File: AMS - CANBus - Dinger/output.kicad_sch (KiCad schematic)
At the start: 7 parts, among them Q3 2N7000, Q4 IRF9Z34NPBF

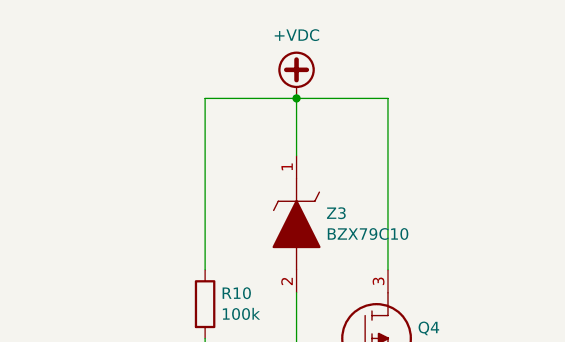
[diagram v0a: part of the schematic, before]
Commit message: initial placement of parts
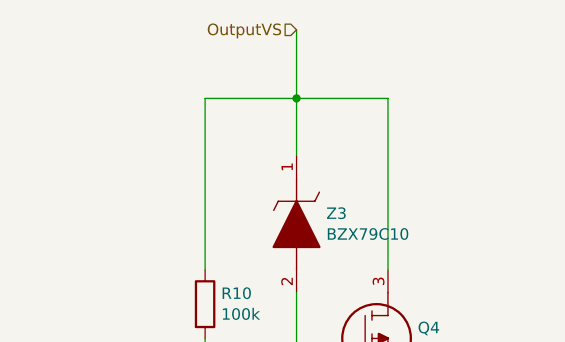
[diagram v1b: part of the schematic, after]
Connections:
- net +VDC renamed OutputVS
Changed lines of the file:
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@@
+	(wire
+		(pts
+			(xy 130.81 54.61) (xy 130.81 62.23)
+		)
+		(stroke
+			(width 0)
+			(type default)
+		)
+	)
 	(wire
 		(pts
@@
 			(width 0)
 			(type default)
+		)
+	)
+	(hierarchical_label "OutputVS"
+		(shape input)
+		(at 130.81 54.61 180)
+		(effects
+			(font
+				(size 1.27 1.27)
+			)
+			(justify right)
 		)
 	)
@@
 					(unit 1)
 				)
-			)
-		)
-	)
-	(symbol
-		(lib_id "power:+VDC")
-		(at 130.81 62.23 0)
-		(unit 1)
-		(exclude_from_sim no)
-		(in_bom yes)
-		(on_board yes)
-		(dnp no)
-		(property "Reference" "#PWR027"
-			(at 130.81 64.77 0)
-			(effects
-				(font
-					(size 1.27 1.27)
-				)
-				(hide yes)
-			)
-		)
-		(property "Value" "+VDC"
-			(at 130.81 55.245 0)
-			(effects
-				(font
-					(size 1.27 1.27)
-				)
-			)
-		)
-		(property "Footprint" ""
-			(at 130.81 62.23 0)
-			(effects
-				(font
-					(size 1.27 1.27)
-				)
-				(hide yes)
-			)
-		)
-		(property "Datasheet" ""
-			(at 130.81 62.23 0)
-			(effects
-				(font
-					(size 1.27 1.27)
-				)
-				(hide yes)
-			)
-		)
-		(property "Description" ""
-			(at 130.81 62.23 0)
-			(effects
-				(font
-					(size 1.27 1.27)
-				)
-				(hide yes)
-			)
-		)
-		(pin "1"
-		)
-		(instances
-			(project "MakeItRain"
-				(path "/6e68f0cd-800e-4167-9553-71fc59da1eeb/00000000-0000-0000-0000-000061506093"
-					(reference "#PWR024")
-					(unit 1)
-				)
-				(path "/6e68f0cd-800e-4167-9553-71fc59da1eeb/00000000-0000-0000-0000-00006158b349"
-					(reference "#PWR027")
-					(unit 1)
-				)
-				(path "/6e68f0cd-800e-4167-9553-71fc59da1eeb/00000000-0000-0000-0000-00006158b83d"
-					(reference "#PWR030")
-					(unit 1)
-				)
-				(path "/6e68f0cd-800e-4167-9553-71fc59da1eeb/00000000-0000-0000-0000-00006158b957"
-					(reference "#PWR033")
-					(unit 1)
-				)
-			)
-			(project "BasicBitch328pThingy"
-				(path "/76196dfb-f920-48e5-a1dc-ea507c9de24d/26dc26ed-3196-4529-9a93-574e99e736ed"
-					(reference "#PWR037")
-					(unit 1)
-				)
-				(path "/76196dfb-f920-48e5-a1dc-ea507c9de24d/612b018a-644d-4608-bec3-996a8f991b06"
-					(reference "#PWR027")
-					(unit 1)
-				)
-				(path "/76196dfb-f920-48e5-a1dc-ea507c9de24d/89689880-8094-4a55-a490-88d5fe271e17"
-					(reference "#PWR039")
-					(unit 1)
-				)
